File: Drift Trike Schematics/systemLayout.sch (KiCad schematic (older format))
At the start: 3 parts

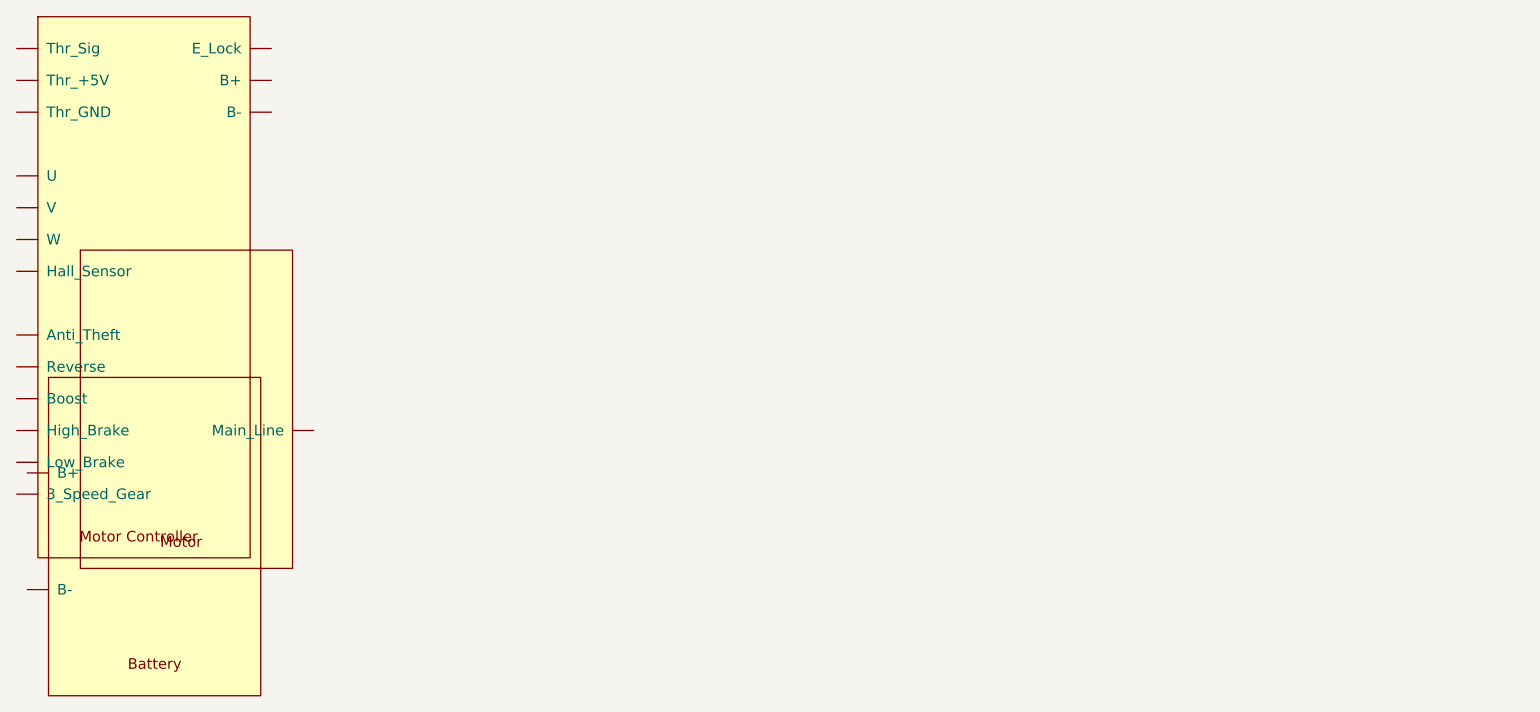
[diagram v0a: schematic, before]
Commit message: Updates
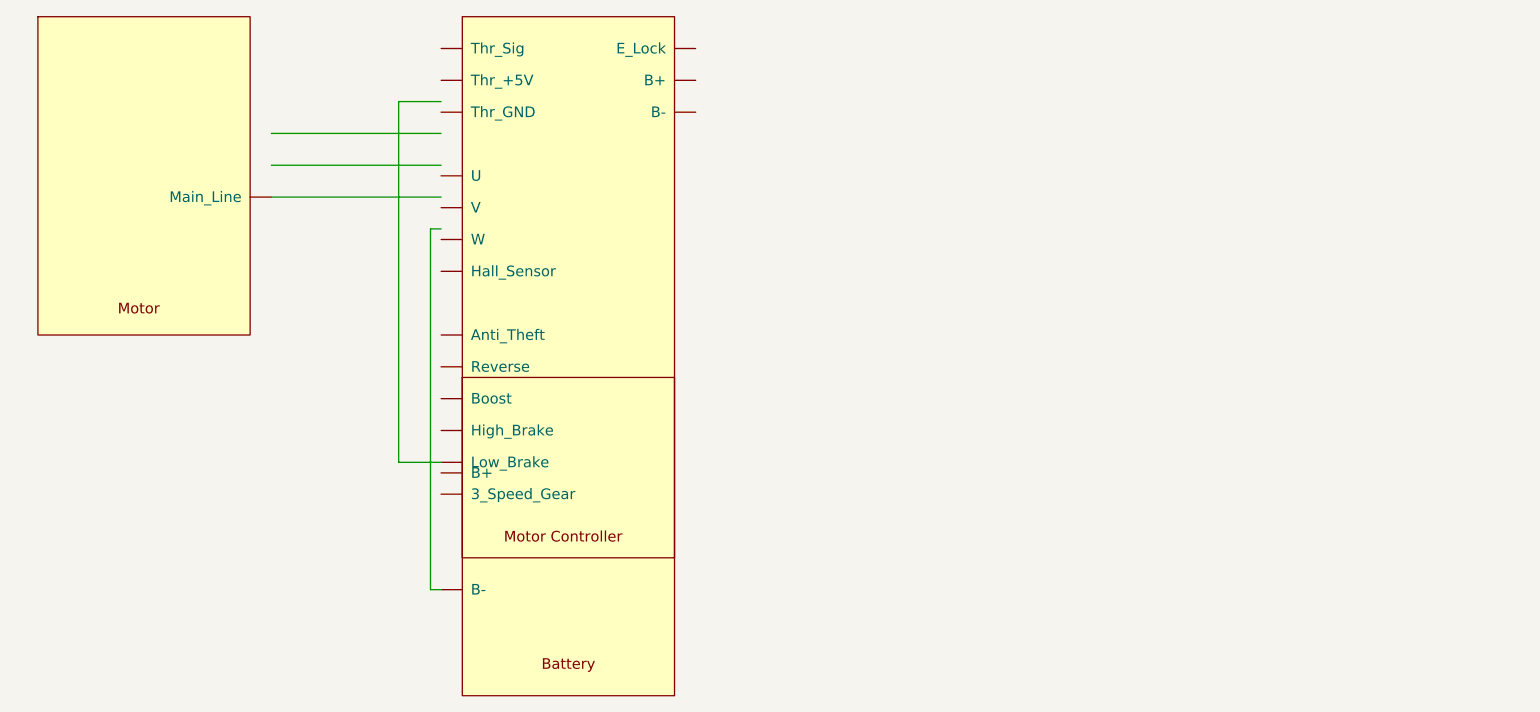
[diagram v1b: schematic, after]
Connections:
- wire segments 0 -> 9
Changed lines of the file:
@@
 L trike_lib:motor_controller U?
 U 1 1 600A3F5E
+P 4500 2000
+F 0 "U?" H 4500 2000 50  0001 C CNN
+F 1 "motor_controller" H 4500 2000 50  0001 C CNN
+F 2 "" H 4500 2000 50  0001 C CNN
+F 3 "" H 4500 2000 50  0001 C CNN
+	1    4500 2000
+	1    0    0    -1
+$EndComp
+$Comp
+L trike_lib:motor U?
+U 1 1 600A5641
 P 2500 2000
 F 0 "U?" H 2500 2000 50  0001 C CNN
-F 1 "motor_controller" H 2500 2000 50  0001 C CNN
+F 1 "motor" H 2500 2000 50  0001 C CNN
 F 2 "" H 2500 2000 50  0001 C CNN
 F 3 "" H 2500 2000 50  0001 C CNN
@@
 $EndComp
 $Comp
-L trike_lib:motor U?
-U 1 1 600A5641
-P 2700 3100
-F 0 "U?" H 2700 3100 50  0001 C CNN
-F 1 "motor" H 2700 3100 50  0001 C CNN
-F 2 "" H 2700 3100 50  0001 C CNN
-F 3 "" H 2700 3100 50  0001 C CNN
-	1    2700 3100
+L trike_lib:battery_block U?
+U 1 1 600A69C3
+P 4500 3700
+F 0 "U?" H 4500 3700 50  0001 C CNN
+F 1 "battery_block" H 4500 3700 50  0001 C CNN
+F 2 "" H 4500 3700 50  0001 C CNN
+F 3 "" H 4500 3700 50  0001 C CNN
+	1    4500 3700
 	1    0    0    -1
 $EndComp
-$Comp
-L trike_lib:battery_block U?
-U 1 1 600A69C3
-P 2550 3700
-F 0 "U?" H 2550 3700 50  0001 C CNN
-F 1 "battery_block" H 2550 3700 50  0001 C CNN
-F 2 "" H 2550 3700 50  0001 C CNN
-F 3 "" H 2550 3700 50  0001 C CNN
-	1    2550 3700
-	1    0    0    -1
-$EndComp
+Wire Wire Line
+	3600 2550 4400 2550
+Wire Wire Line
+	3600 2700 4400 2700
+Wire Wire Line
+	3600 2850 4400 2850
+Wire Wire Line
+	4400 4700 4350 4700
+Wire Wire Line
+	4400 3000 4350 3000
+Wire Wire Line
+	4350 3000 4350 4700
+Wire Wire Line
+	4400 4100 4200 4100
+Wire Wire Line
+	4200 4100 4200 2400
+Wire Wire Line
+	4200 2400 4400 2400
 $EndSCHEMATC

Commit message: Updates
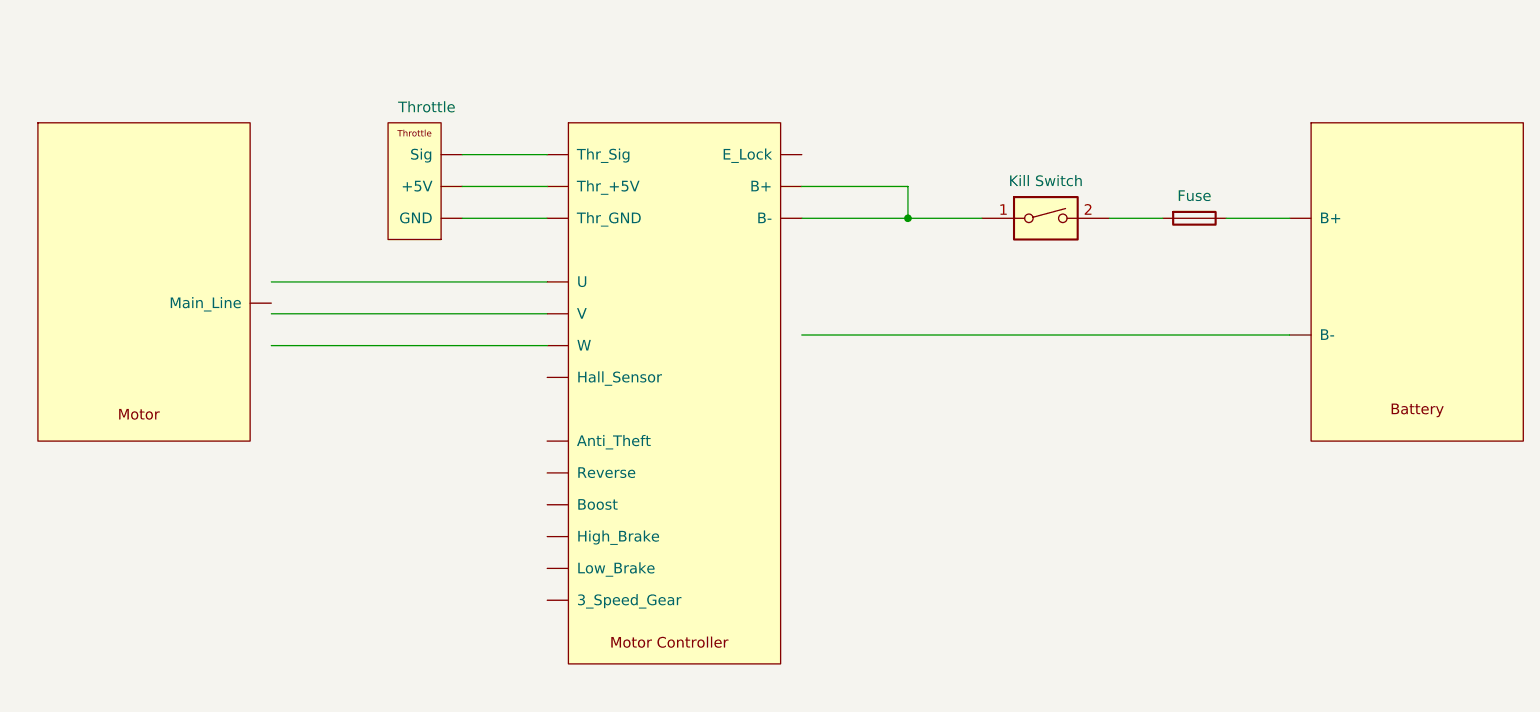
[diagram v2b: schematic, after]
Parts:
- added F: Fuse, symbol Device:Fuse
- added SW: Kill Switch, symbol Switch:SW_DIP_x01
- added U: Throttle, symbol trike_lib:Throttle
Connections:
- wire segments 9 -> 13
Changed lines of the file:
@@
 $EndDescr
+$Comp
+L trike_lib:battery_block U?
+U 1 1 600A69C3
+P 8500 2500
+F 0 "U?" H 8500 2500 50  0001 C CNN
+F 1 "battery_block" H 8500 2500 50  0001 C CNN
+F 2 "" H 8500 2500 50  0001 C CNN
+F 3 "" H 8500 2500 50  0001 C CNN
+	1    8500 2500
+	1    0    0    -1
+$EndComp
+$Comp
+L Switch:SW_DIP_x01 SW
+U 1 1 605441B3
+P 7250 2950
+F 0 "SW" H 7250 3217 50  0001 C CNN
+F 1 "Kill Switch" H 7250 3125 50  0000 C CNN
+F 2 "" H 7250 2950 50  0001 C CNN
+F 3 "~" H 7250 2950 50  0001 C CNN
+	1    7250 2950
+	1    0    0    -1
+$EndComp
 $Comp
 L trike_lib:motor_controller U?
 U 1 1 600A3F5E
-P 4500 2000
-F 0 "U?" H 4500 2000 50  0001 C CNN
-F 1 "motor_controller" H 4500 2000 50  0001 C CNN
-F 2 "" H 4500 2000 50  0001 C CNN
-F 3 "" H 4500 2000 50  0001 C CNN
-	1    4500 2000
+P 5000 2500
+F 0 "U?" H 5000 2500 50  0001 C CNN
+F 1 "motor_controller" H 5000 2500 50  0001 C CNN
+F 2 "" H 5000 2500 50  0001 C CNN
+F 3 "" H 5000 2500 50  0001 C CNN
+	1    5000 2500
 	1    0    0    -1
 $EndComp
 $Comp
+L Device:Fuse F
+U 1 1 6055BA66
+P 7950 2950
+F 0 "F" V 7753 2950 50  0001 C CNN
+F 1 "Fuse" V 7845 2950 50  0000 C CNN
+F 2 "" V 7880 2950 50  0001 C CNN
+F 3 "~" H 7950 2950 50  0001 C CNN
+	1    7950 2950
+	0    1    1    0
+$EndComp
+Wire Wire Line
+	8400 2950 8100 2950
+Wire Wire Line
+	7550 2950 7800 2950
+Wire Wire Line
+	6100 2950 6600 2950
+Wire Wire Line
+	6100 2800 6600 2800
+Wire Wire Line
+	6600 2800 6600 2950
+Connection ~ 6600 2950
+Wire Wire Line
+	6600 2950 6950 2950
+Wire Wire Line
+	6100 3500 8400 3500
+Wire Wire Line
+	3600 3550 4900 3550
+Wire Wire Line
+	4900 3400 3600 3400
+Wire Wire Line
+	4900 3250 3600 3250
+$Comp
 L trike_lib:motor U?
 U 1 1 600A5641
-P 2500 2000
-F 0 "U?" H 2500 2000 50  0001 C CNN
-F 1 "motor" H 2500 2000 50  0001 C CNN
-F 2 "" H 2500 2000 50  0001 C CNN
-F 3 "" H 2500 2000 50  0001 C CNN
-	1    2500 2000
+P 2500 2500
+F 0 "U?" H 2500 2500 50  0001 C CNN
+F 1 "motor" H 2500 2500 50  0001 C CNN
+F 2 "" H 2500 2500 50  0001 C CNN
+F 3 "" H 2500 2500 50  0001 C CNN
+	1    2500 2500
 	1    0    0    -1
 $EndComp
 $Comp
-L trike_lib:battery_block U?
-U 1 1 600A69C3
-P 4500 3700
-F 0 "U?" H 4500 3700 50  0001 C CNN
-F 1 "battery_block" H 4500 3700 50  0001 C CNN
-F 2 "" H 4500 3700 50  0001 C CNN
-F 3 "" H 4500 3700 50  0001 C CNN
-	1    4500 3700
+L trike_lib:Throttle U
+U 1 1 60566AFA
+P 4150 2500
+F 0 "U" H 4333 2665 50  0001 C CNN
+F 1 "Throttle" H 4333 2573 50  0000 C CNN
+F 2 "" H 4550 1950 50  0001 C CNN
+F 3 "" H 4550 1950 50  0001 C CNN
+	1    4150 2500
 	1    0    0    -1
 $EndComp
 Wire Wire Line
-	3600 2550 4400 2550
+	4500 2650 4900 2650
 Wire Wire Line
-	3600 2700 4400 2700
+	4500 2950 4900 2950
 Wire Wire Line
-	3600 2850 4400 2850
-Wire Wire Line
-	4400 4700 4350 4700
-Wire Wire Line
-	4400 3000 4350 3000
-Wire Wire Line
-	4350 3000 4350 4700
-Wire Wire Line
-	4400 4100 4200 4100
-Wire Wire Line
-	4200 4100 4200 2400
-Wire Wire Line
-	4200 2400 4400 2400
+	4500 2800 4900 2800
 $EndSCHEMATC
